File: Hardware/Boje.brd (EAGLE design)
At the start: 18 x 18 mm, 11 parts, among them IC1 TINY13V-10PU, J1 POWER, J2 Free, J3 SWITCH

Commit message: Part Change
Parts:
- IC1: value TINY13V-10PU -> AT-TINY85V
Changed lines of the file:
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@@
 </autorouter>
 <elements>
-<element name="IC1" library="atmel" package="DIL08" value="TINY13V-10PU" x="10.00125" y="6.82625" smashed="yes">
+<element name="IC1" library="atmel" package="DIL08" value="AT-TINY85V" x="10.00125" y="6.82625" smashed="yes">
 <attribute name="MF" value="" x="10.00125" y="6.82625" size="1.778" layer="27" display="off"/>
 <attribute name="OC_FARNELL" value="9171576" x="10.00125" y="6.82625" size="1.778" layer="27" display="off"/>

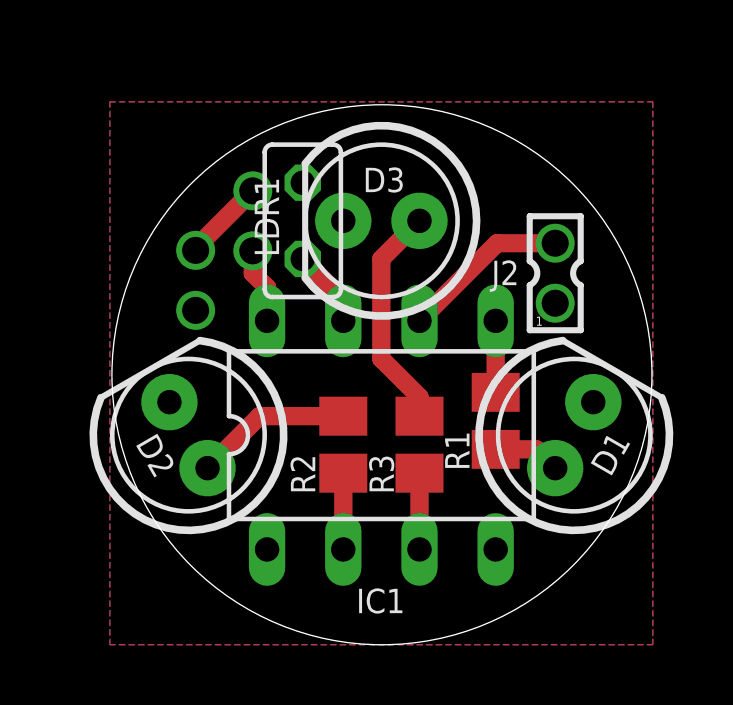
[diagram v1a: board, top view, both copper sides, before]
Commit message: New Layout
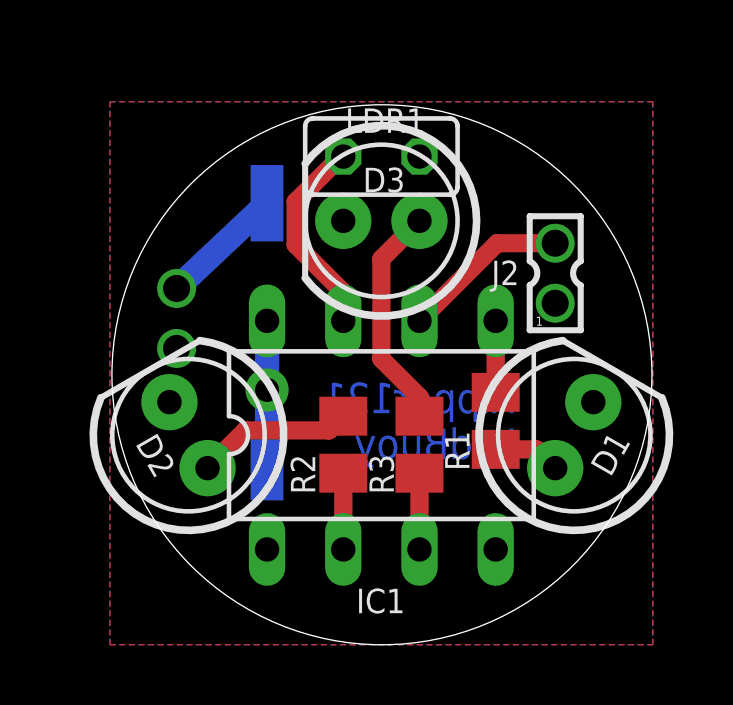
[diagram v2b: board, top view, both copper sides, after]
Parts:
- removed J3: SWITCH, con-garry:332-02
- added DRILEGEND: (no value), drilegend:DRILEGEND
- added SW1: SWS001, smd-special:SMS-001
- D1: value (none) -> LED0
- D2: value (none) -> LED1
- D3: value (none) -> LED2
- moved LDR1 3.38 mm to (10.0, 16.1), turned to 180 degrees
- moved J1 1.42 mm to (3.17, 10.7)
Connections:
- removed net VCC-5V: IC1.8, J3.2
- new net VCC: IC1.8, SW1.1
- net N$1: now also SW1.2; no longer J3.1
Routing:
- net VCC: track 0.00 -> 4.71 mm, vias 0 -> 1
- net N$14: track 2.62 -> 6.84 mm
- net VCC-5V: track 2.53 -> 0.00 mm
- net N$1: track 2.77 -> 4.15 mm
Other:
- board text added: "01-16"
- board text added: "D1"
- board text added: "D2"
- board text added: "D3"
- board text added: "IC1"
- board text added: "J1"
- board text added: "J2"
- board text added: "J3"
- board text added: "LAYER-STACK"
- board text added: "LDR1"
- board text added: "R1"
- board text added: "R2"
- board text added: "R3"
- board text added: "Ripper121 LedBuoy"

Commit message: Gerber
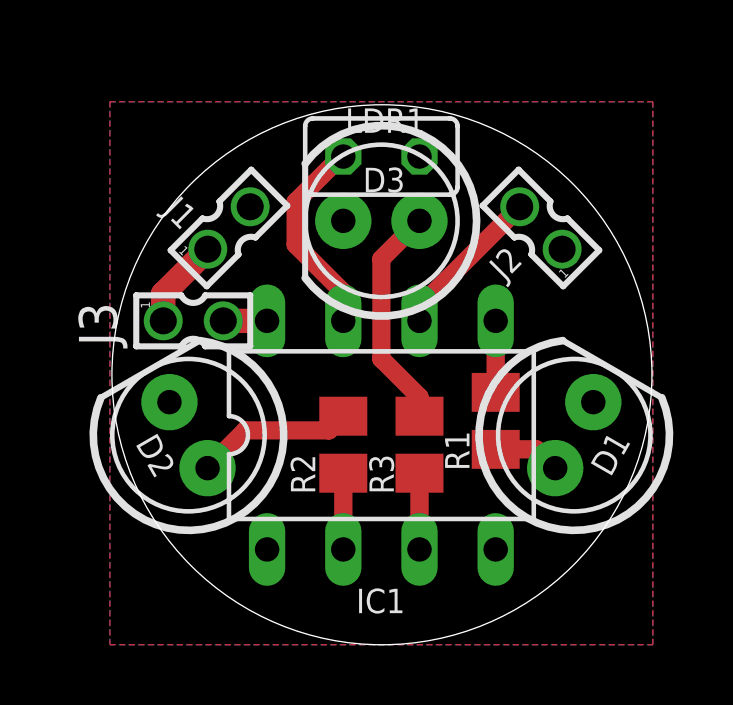
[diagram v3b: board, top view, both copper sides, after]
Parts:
- removed SW1: SWS001, smd-special:SMS-001
- added J3: SWITCH, con-garry:332-02
- moved J1 3.49 mm to (4.92, 13.7), flipped to the top, turned to 315 degrees
- moved J2 1.58 mm to (15.3, 13.7), turned to 45 degrees
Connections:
- net N$1: now also J3.1; no longer SW1.2
- net VCC: now also J3.2; no longer SW1.1
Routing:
- net VCC: track 4.71 -> 1.46 mm, vias 1 -> 0
- net N$1: track 4.15 -> 3.00 mm
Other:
- board text removed: "Ripper121 LedBuoy"
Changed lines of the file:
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@@
 <layers>
 <layer number="1" name="Top" color="4" fill="1" visible="yes" active="yes"/>
-<layer number="16" name="Bottom" color="1" fill="1" visible="yes" active="yes"/>
+<layer number="16" name="Bottom" color="1" fill="1" visible="no" active="yes"/>
 <layer number="17" name="Pads" color="2" fill="1" visible="yes" active="yes"/>
 <layer number="18" name="Vias" color="2" fill="1" visible="yes" active="yes"/>
@@
 <layer number="20" name="Dimension" color="15" fill="1" visible="yes" active="yes"/>
 <layer number="21" name="tPlace" color="7" fill="1" visible="yes" active="yes"/>
-<layer number="22" name="bPlace" color="7" fill="1" visible="yes" active="yes"/>
+<layer number="22" name="bPlace" color="7" fill="1" visible="no" active="yes"/>
 <layer number="23" name="tOrigins" color="15" fill="1" visible="yes" active="yes"/>
-<layer number="24" name="bOrigins" color="15" fill="1" visible="yes" active="yes"/>
-<layer number="25" name="tNames" color="7" fill="1" visible="no" active="yes"/>
+<layer number="24" name="bOrigins" color="15" fill="1" visible="no" active="yes"/>
+<layer number="25" name="tNames" color="7" fill="1" visible="yes" active="yes"/>
 <layer number="26" name="bNames" color="7" fill="1" visible="no" active="yes"/>
 <layer number="27" name="tValues" color="7" fill="1" visible="no" active="yes"/>
 <layer number="28" name="bValues" color="7" fill="1" visible="no" active="yes"/>
 <layer number="29" name="tStop" color="7" fill="3" visible="yes" active="yes"/>
-<layer number="30" name="bStop" color="7" fill="6" visible="yes" active="yes"/>
+<layer number="30" name="bStop" color="7" fill="6" visible="no" active="yes"/>
 <layer number="31" name="tCream" color="7" fill="4" visible="yes" active="yes"/>
-<layer number="32" name="bCream" color="7" fill="5" visible="yes" active="yes"/>
+<layer number="32" name="bCream" color="7" fill="5" visible="no" active="yes"/>
 <layer number="33" name="tFinish" color="6" fill="3" visible="no" active="yes"/>
 <layer number="34" name="bFinish" color="6" fill="6" visible="no" active="yes"/>
@@
 <layer number="38" name="bTest" color="7" fill="1" visible="no" active="yes"/>
 <layer number="39" name="tKeepout" color="4" fill="11" visible="yes" active="yes"/>
-<layer number="40" name="bKeepout" color="1" fill="11" visible="yes" active="yes"/>
+<layer number="40" name="bKeepout" color="1" fill="11" visible="no" active="yes"/>
 <layer number="41" name="tRestrict" color="4" fill="10" visible="yes" active="yes"/>
-<layer number="42" name="bRestrict" color="1" fill="10" visible="yes" active="yes"/>
+<layer number="42" name="bRestrict" color="1" fill="10" visible="no" active="yes"/>
 <layer number="43" name="vRestrict" color="2" fill="10" visible="no" active="yes"/>
 <layer number="44" name="Drills" color="7" fill="1" visible="no" active="yes"/>
@@
 <layer number="50" name="dxf" color="7" fill="1" visible="no" active="no"/>
 <layer number="51" name="tDocu" color="7" fill="1" visible="yes" active="yes"/>
-<layer number="52" name="bDocu" color="7" fill="1" visible="yes" active="yes"/>
+<layer number="52" name="bDocu" color="7" fill="1" visible="no" active="yes"/>
 <layer number="53" name="tGND_GNDA" color="7" fill="1" visible="no" active="no"/>
 <layer number="54" name="bGND_GNDA" color="7" fill="1" visible="no" active="no"/>
@@
 <wire x1="5.207" y1="13.478" x2="6.223" y2="12.462" width="0.1016" layer="145"/>
 <wire x1="6.223" y1="13.478" x2="5.207" y2="12.462" width="0.1016" layer="145"/>
-<text x="14.525625" y="6.0325" size="1.016" layer="16" font="vector" rot="MR0">Ripper121
-LedBuoy</text>
 </plain>
 <attributes>
@@
 <attribute name="VALUE" x="12.41425" y="18.907125" size="1.27" layer="27" ratio="10" rot="R180"/>
 </element>
-<element name="J1" library="con-garry" package="332-02" value="POWER" x="3.175" y="10.715625" smashed="yes" rot="MR180">
-<attribute name="NAME" x="1.205625" y="11.90625" size="0.8128" layer="26" rot="MR180"/>
-<attribute name="VALUE" x="2.555" y="8.175625" size="1.27" layer="28" rot="MR180"/>
-</element>
-<element name="J2" library="con-garry" package="332-02" value="Free" x="15.795625" y="12.22375" smashed="yes">
-<attribute name="NAME" x="13.6675" y="11.826875" size="0.8128" layer="25"/>
-<attribute name="VALUE" x="15.175625" y="14.76375" size="1.27" layer="27"/>
+<element name="J1" library="con-garry" package="332-02" value="POWER" x="4.92125" y="13.731875" smashed="yes" rot="R315">
+<attribute name="NAME" x="2.686790625" y="14.282534375" size="0.8128" layer="25" rot="R315"/>
+<attribute name="VALUE" x="6.27889375" y="15.96633125" size="1.27" layer="27" rot="R315"/>
+</element>
+<element name="J2" library="con-garry" package="332-02" value="Free" x="15.319375" y="13.731875" smashed="yes" rot="R45">
+<attribute name="NAME" x="14.09519375" y="11.946428125" size="0.8128" layer="25" rot="R45"/>
+<attribute name="VALUE" x="13.084915625" y="15.08951875" size="1.27" layer="27" rot="R45"/>
 </element>
 <element name="DRILEGEND" library="drilegend" package="DRILEGEND" value="" x="-4.945178125" y="-9.825"/>
-<element name="SW1" library="smd-special" package="SMS-001" value="SWS001" x="6.19125" y="10.239375" rot="MR0"/>
+<element name="J3" library="con-garry" package="332-02" value="SWITCH" x="3.730625" y="10.63625" rot="R270"/>
 </elements>
 <signals>
@@
 <signal name="VCC">
 <contactref element="IC1" pad="8"/>
-<contactref element="SW1" pad="1"/>
-<wire x1="6.19125" y1="5.921375" x2="6.19125" y2="8.334375" width="0.8128" layer="16"/>
-<wire x1="6.19125" y1="8.334375" x2="6.19125" y2="10.63625" width="0.8128" layer="16"/>
-<via x="6.19125" y="8.334375" extent="1-16" drill="0.8" shape="octagon"/>
+<contactref element="J3" pad="2"/>
+<wire x1="4.730625" y1="10.63625" x2="6.19125" y2="10.63625" width="0.8128" layer="1"/>
 </signal>
 <signal name="N$13">
@@
 <contactref element="IC1" pad="6"/>
 <contactref element="J2" pad="2"/>
-<wire x1="11.27125" y1="10.63625" x2="13.85875" y2="13.22375" width="0.6096" layer="1"/>
-<wire x1="13.85875" y1="13.22375" x2="15.795625" y2="13.22375" width="0.6096" layer="1"/>
+<wire x1="11.27125" y1="10.63625" x2="11.27125" y2="11.097965625" width="0.6096" layer="1"/>
+<wire x1="11.27125" y1="11.097965625" x2="14.612265625" y2="14.43898125" width="0.6096" layer="1"/>
 </signal>
 <signal name="N$1">
 <contactref element="J1" pad="1"/>
-<contactref element="SW1" pad="2"/>
-<wire x1="3.175" y1="11.715625" x2="3.175" y2="11.718925" width="0.8128" layer="16"/>
-<wire x1="3.175" y1="11.718925" x2="6.19125" y2="14.557375" width="0.8128" layer="16"/>
+<contactref element="J3" pad="1"/>
+<wire x1="4.214140625" y1="13.024765625" x2="2.730625" y2="11.54125" width="0.8128" layer="1"/>
+<wire x1="2.730625" y1="11.54125" x2="2.730625" y2="10.63625" width="0.8128" layer="1"/>
 </signal>
 </signals>
@@
 </board>
 </drawing>
-<compatibility>
-<note version="6.3" minversion="6.2.2" severity="warning">
-Since Version 6.2.2 text objects can contain more than one line,
-which will not be processed correctly with this version.
-</note>
-</compatibility>
 </eagle>

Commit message: New PCB Layout
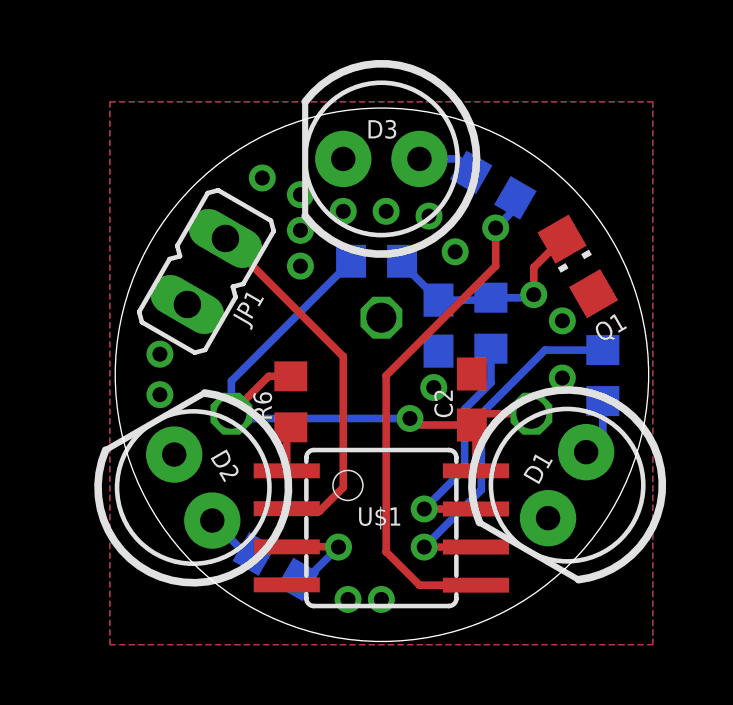
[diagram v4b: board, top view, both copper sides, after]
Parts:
- removed DRILEGEND: (no value), drilegend:DRILEGEND
- removed IC1: AT-TINY85V, atmel:DIL08
- removed J1: POWER, con-garry:332-02
- removed J2: Free, con-garry:332-02
- removed J3: SWITCH, con-garry:332-02
- removed LDR1: LDR, rcl:V526-0
- added C1, C2: 100nF, rcl:C0603
- added G1: S8401-46, battery_holder:CR2032V
- added JP1: (no value), jumper:JP1
- added Q1: PT15-21C/TR8, SparkFun-DiscreteSemi:PT17-21C-L41-TR8
- added R4, R5: 1k, rcl:R0603
- added R6: 100k, rcl:R0603
- added U$1: TINY85-20SU, avr-6:SOIC8
- R1, R2, R3: value 68 -> 120; device resistor:M2012 -> rcl:R0603
- moved R3 8.99 mm to (13.7, 15.2), flipped to the bottom, turned to 210 degrees
- moved R2 4.65 mm to (6.49, 2.44), flipped to the bottom, turned to 210 degrees
- moved R1 3.88 mm to (17.4, 8.81), flipped to the bottom
- moved D3 2.06 mm to (10.0, 16.0)
- moved D2 1.75 mm to (3.73, 5.08)
- moved D1 1.68 mm to (16.2, 5.16), turned to 240 degrees
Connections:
- removed net N$11: IC1.3, R3.2
- removed net N$12: IC1.2, R2.2
- removed net N$13: IC1.5, R1.2
- removed net N$14: IC1.7, LDR1.2
- removed net N$7: IC1.6, J2.2
- new net FREE: JP1.1, U$1.2
- new net LED0: R1.2, U$1.6
- new net LED1: R2.2, U$1.3
- new net LED2: R3.2, U$1.5
- new net LIGHT: R5.1, U$1.7
- new net RESET: R6.1, U$1.1
- net GND: now also C1.1, C2.2, G1.-, JP1.2, Q1.E, U$1.4; no longer IC1.4, J1.2, J2.1, LDR1.1
- net N$1: now also C1.2, Q1.C, R4.1, R5.2; no longer J1.1, J3.1
- net VCC: now also C2.1, G1.+0, G1.+1, R4.2, R6.2, U$1.8; no longer IC1.8, J3.2
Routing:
- net VCC: track 1.46 -> 21.1 mm, vias 0 -> 1
- net LED2: track 0.00 -> 17.0 mm, vias 0 -> 1
- net FREE: track 0.00 -> 12.2 mm
- net LED0: track 0.00 -> 11.9 mm, vias 0 -> 1
- net LIGHT: track 0.00 -> 7.99 mm, vias 0 -> 1
- net N$14: track 6.84 -> 0.00 mm
- net N$6: track 7.56 -> 1.91 mm
- net N$7: track 5.19 -> 0.00 mm
- net N$1: track 3.00 -> 7.29 mm, vias 0 -> 1
- net LED1: track 0.00 -> 3.53 mm, vias 0 -> 1
- net N$5: track 5.24 -> 1.85 mm
- net N$12: track 2.54 -> 0.00 mm
- net N$11: track 2.54 -> 0.00 mm
- net N$13: track 2.38 -> 0.00 mm
- net RESET: track 0.00 -> 1.51 mm
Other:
- board size 18 x 18 mm -> 17.8 x 17.8 mm
- board text removed: "01-16"
- board text removed: "LAYER-STACK"
